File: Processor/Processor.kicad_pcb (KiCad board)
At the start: 2 copper layers, 100 x 100 mm, 44 parts, among them J1 Buss, J2 L2, J3 L3, U1 MC6800, U10 74LS573, U11 74LS573, U2 74LS74, U3 74LS00, U4 74LS245, U5 74LS573, U6 74LS138, U7 GAL20V8, U8 74LS04, U9 74LS573, Y1 2.0MHz

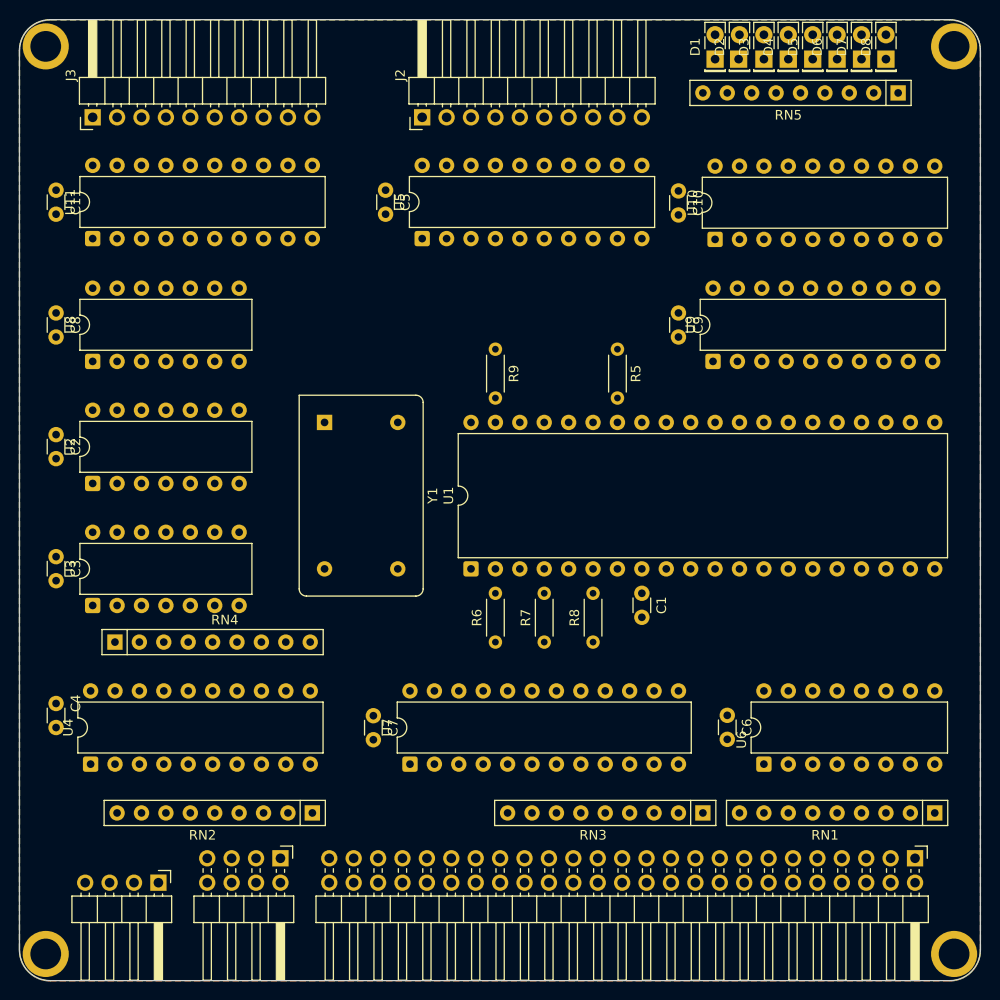
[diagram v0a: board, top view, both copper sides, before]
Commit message: a bunch of stuff
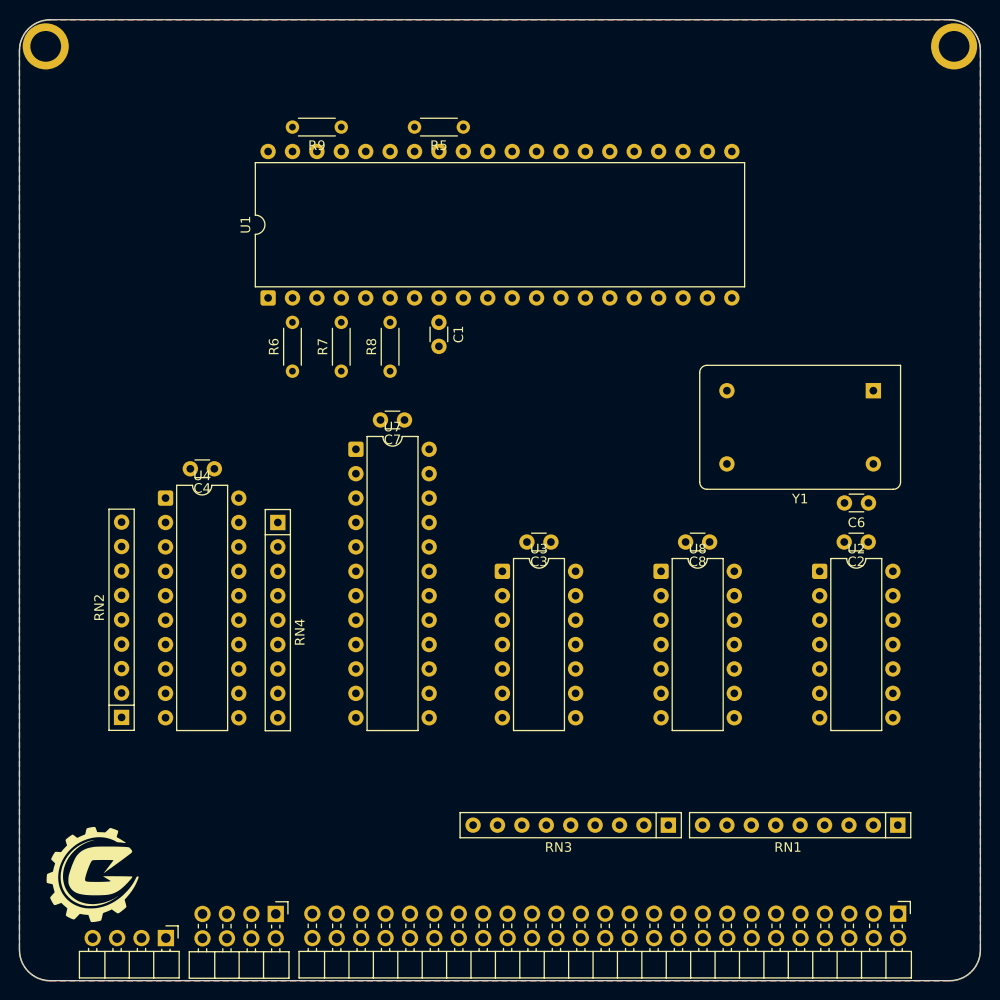
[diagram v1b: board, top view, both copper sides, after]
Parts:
- removed C10, C11, C5, C9: 100n, Capacitor_THT:C_Disc_D3.0mm_W1.6mm_P2.50mm
- removed D1: S0, LED_THT:LED_Rectangular_W5.0mm_H2.0mm
- removed D2: S1, LED_THT:LED_Rectangular_W5.0mm_H2.0mm
- removed D3: S2, LED_THT:LED_Rectangular_W5.0mm_H2.0mm
- removed D4: S3, LED_THT:LED_Rectangular_W5.0mm_H2.0mm
- removed D5: S4, LED_THT:LED_Rectangular_W5.0mm_H2.0mm
- removed D6: S5, LED_THT:LED_Rectangular_W5.0mm_H2.0mm
- removed D7: S6, LED_THT:LED_Rectangular_W5.0mm_H2.0mm
- removed D8: S7, LED_THT:LED_Rectangular_W5.0mm_H2.0mm
- removed J2: L2, Connector_PinHeader_2.54mm:PinHeader_1x10_P2.54mm_Horizontal
- removed J3: L3, Connector_PinHeader_2.54mm:PinHeader_1x10_P2.54mm_Horizontal
- removed RN5: 220Ω, Resistor_THT:R_Array_SIP9
- removed U10, U11, U5, U9: 74LS573, Package_DIP:DIP-20_W7.62mm
- removed U6: 74LS138, Package_DIP:DIP-16_W7.62mm
- added G1: Logo, 0-Footprints:Crank, F.Cu at (32.7, 114.0)
- U7: value GAL20V8 -> GAL22V10
- moved C2 85.3 mm to (113.3, 79.4), turned to 180 degrees
- moved U2 76.2 mm to (108.3, 82.4), turned to 0 degrees
- moved C8 72.1 mm to (96.8, 79.4), turned to 180 degrees
- moved U8 63.1 mm to (91.8, 82.4), turned to 0 degrees
- moved Y1 57.2 mm to (113.9, 63.6), turned to 180 degrees
- moved C3 51.5 mm to (80.3, 79.4), turned to 180 degrees
- moved U3 42.8 mm to (75.3, 82.4), turned to 0 degrees
- moved R6 35.2 mm to (53.4, 61.6)
- moved C1 35.2 mm to (68.7, 56.5)
- moved R7 35.2 mm to (58.5, 61.6)
- moved R8 35.2 mm to (63.6, 61.6)
- moved U1 35.2 mm to (50.9, 54.0)
- moved U7 33.2 mm to (60.0, 69.7), turned to 0 degrees
- moved C7 30.9 mm to (65.1, 66.7), turned to 180 degrees
- moved C4 29.5 mm to (45.3, 71.7), turned to 180 degrees
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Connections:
- J1 pad 10: BANK_0 -> unconnected-(J1-Pad10)
- J1 pad 12: BANK_1 -> unconnected-(J1-Pad12)
- J1 pad 14: BANK_2 -> unconnected-(J1-Pad14)
- J1 pad 16: BANK_3 -> unconnected-(J1-Pad16)
- J1 pad 18: BANK_4 -> unconnected-(J1-Pad18)
- J1 pad 20: BANK_5 -> unconnected-(J1-Pad20)
- J1 pad 22: BANK_6 -> unconnected-(J1-Pad22)
- J1 pad 24: BANK_7 -> unconnected-(J1-Pad24)
- J1 pad 44: Φ2 -> unconnected-(J1-Pad44)
- J1 pad B3: unconnected-(J1-PadB3) -> Φ2
- U3 pad 10: Net-(U6-O1) -> GND
- U3 pad 11: LOAD_0 -> unconnected-(U3-Pad11)
- U3 pad 12: Net-(U6-O0) -> GND
- U3 pad 13: Net-(U6-O0) -> GND
- U3 pad 8: LOAD_1 -> unconnected-(U3-Pad8)
- U3 pad 9: Net-(U6-O1) -> GND
- U7 pad 10: A12 -> A8
- U7 pad 11: A11 -> GND
- U7 pad 13: A10 -> GND
- U7 pad 14: A9 -> GND
- U7 pad 17: ~{LATCH_SEL} -> GND
- U7 pad 18: BUS_OK -> GND
- U7 pad 19: ~{IO_SEL} -> BUS_OK
- U7 pad 20: ~{BANK_SEL} -> ~{IO_SEL}
- U7 pad 21: ~{ROM_SEL} -> ~{BANK_SEL}
- U7 pad 22: ~{RAM_SEL} -> ~{ROM_SEL}
- U7 pad 23: A8 -> ~{RAM_SEL}
- U7 pad 3: GND -> A15
- U7 pad 4: GND -> A14
- U7 pad 5: GND -> A13
- U7 pad 6: GND -> A12
- U7 pad 7: A15 -> A11
- U7 pad 8: A14 -> A10
- U7 pad 9: A13 -> A9
- U8 pad 10: LOAD_2 -> unconnected-(U8-Pad10)
- U8 pad 11: Net-(U6-O2) -> GND
- U8 pad 12: LOAD_3 -> unconnected-(U8-Pad12)
- U8 pad 13: Net-(U6-O3) -> GND

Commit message: ordered v01 of the cpu
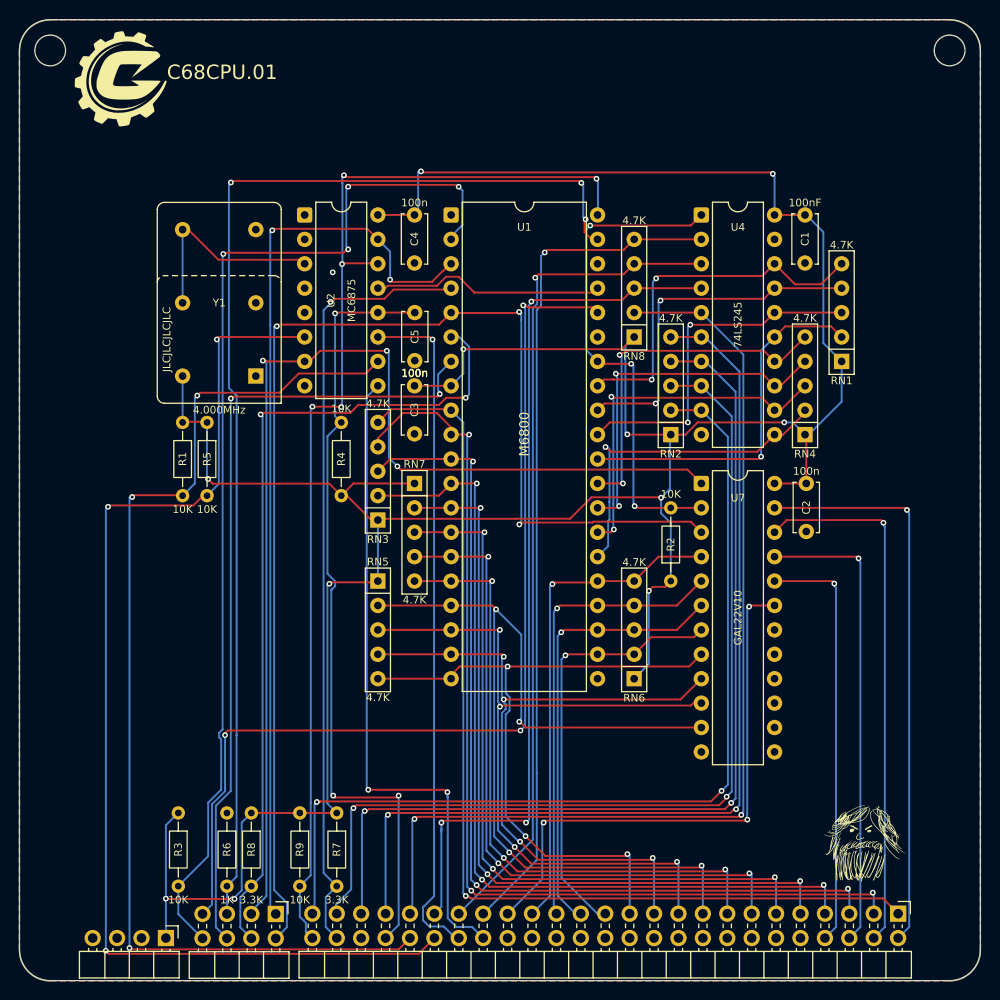
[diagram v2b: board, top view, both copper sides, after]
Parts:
- removed C6, C7, C8: 100n, Capacitor_THT:C_Disc_D3.0mm_W1.6mm_P2.50mm
- removed the R6 at (53.4, 61.6)
- removed U3: 74LS00, Package_DIP:DIP-14_W7.62mm
- removed U8: 74LS04, Package_DIP:DIP-14_W7.62mm
- added C5: 100n, 0-Footprints:C_Disc_D5.0mm_W2.5mm_P5.00mm, F.Cu at (66.1, 55.5)
- added G2: Crankery, 0-Footprints:crankery_small, F.Cu at (112.7, 110.8)
- added G3: Motorola, 0-Footprints:Motorola, B.Cu at (69.3, 31.0)
- added G4: Crank, 0-Footprints:Crank, B.Cu at (103.4, 31.1)
- added R1: 10K, 0-Footprints:R_Axial_DIN0204_L3.6mm_D1.6mm_P7.62mm_Horizontal, F.Cu at (42.0, 66.9)
- added R2: 10K, 0-Footprints:R_Axial_DIN0204_L3.6mm_D1.6mm_P7.62mm_Horizontal, F.Cu at (92.8, 83.4)
- added R3: 10K, 0-Footprints:R_Axial_DIN0204_L3.6mm_D1.6mm_P7.62mm_Horizontal, F.Cu at (41.5, 107.5)
- added R4: 10K, 0-Footprints:R_Axial_DIN0204_L3.6mm_D1.6mm_P7.62mm_Horizontal, F.Cu at (58.5, 74.5)
- added R9: 10K, 0-Footprints:R_Axial_DIN0204_L3.6mm_D1.6mm_P7.62mm_Horizontal, F.Cu at (54.2, 107.5)
- added RN5: 4.7K, 0-Footprints:R_Array_SIP5, F.Cu at (62.3, 83.4)
- added RN6: 4.7K, 0-Footprints:R_Array_SIP5, F.Cu at (89.0, 93.6)
- added RN7: 4.7K, 0-Footprints:R_Array_SIP5, F.Cu at (66.1, 73.3)
- added RN8: 4.7K, 0-Footprints:R_Array_SIP5, F.Cu at (89.0, 58.0)
- C1: value 100n -> 100nF; footprint Capacitor_THT:C_Disc_D3.0mm_W1.6mm_P2.50mm -> 0-Footprints:C_Disc_D5.0mm_W2.5mm_P5.00mm
- C2, C3, C4: footprint Capacitor_THT:C_Disc_D3.0mm_W1.6mm_P2.50mm -> 0-Footprints:C_Disc_D5.0mm_W2.5mm_P5.00mm
- G1: value Logo -> Crank
- R5, R7, R8: footprint Resistor_THT:R_Axial_DIN0204_L3.6mm_D1.6mm_P5.08mm_Horizontal -> 0-Footprints:R_Axial_DIN0204_L3.6mm_D1.6mm_P7.62mm_Horizontal
- R6: renamed from R9; footprint Resistor_THT:R_Axial_DIN0204_L3.6mm_D1.6mm_P5.08mm_Horizontal -> 0-Footprints:R_Axial_DIN0204_L3.6mm_D1.6mm_P7.62mm_Horizontal
- RN1, RN2, RN3, RN4: footprint Resistor_THT:R_Array_SIP9 -> 0-Footprints:R_Array_SIP5
- U1: value MC6800 -> M6800; footprint Package_DIP:DIP-40_W15.24mm -> 0-Footprints:DIP-40_W15.24mm
- U2: value 74LS74 -> MC6875; footprint Package_DIP:DIP-14_W7.62mm -> 0-Footprints:DIP-16_W7.62mm
- U4: footprint Package_DIP:DIP-20_W7.62mm -> 0-Footprints:DIP-20_W7.62mm
- U7: footprint Package_DIP:DIP-24_W7.62mm -> 0-Footprints:DIP-24_W7.62mm
- Y1: value 2.0MHz -> 4.000MHz; footprint Oscillator:Oscillator_DIP-14 -> 0-Footprints:Oscillator_DIP-14
- moved G1 82.9 mm to (35.6, 31.2)
- moved R6 72.4 mm to (46.6, 107.5), turned to -90 degrees
- moved U2 65.2 mm to (54.7, 45.3)
- moved RN2 64.3 mm to (92.8, 68.2)
- moved Y1 64.3 mm to (49.6, 62.1), turned to 90 degrees
- moved U4 63.1 mm to (96.0, 45.3)
- moved RN4 55.6 mm to (106.8, 68.2), turned to 90 degrees
- moved RN1 48.6 mm to (110.6, 60.6), turned to 90 degrees
- moved R8 48.2 mm to (49.1, 107.5), turned to -90 degrees
- moved R7 46.0 mm to (58.0, 107.5), turned to -90 degrees
- moved RN3 43.8 mm to (62.3, 77.1), turned to 90 degrees
- moved R5 40.7 mm to (44.5, 66.9), turned to -90 degrees
- moved C1 38.6 mm to (106.8, 50.3), turned to 90 degrees
- moved U7 36.1 mm to (96.0, 73.3)
- moved C4 29.9 mm to (66.1, 50.3), turned to 90 degrees
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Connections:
- net 2.0MHz renamed Net-(U2-EXT_IN)
- C1 pad 1: +5V -> GND
- C1 pad 2: GND -> +5V
- C2 pad 1: +5V -> GND
- C2 pad 2: GND -> +5V
- C3 pad 1: +5V -> GND
- C3 pad 2: GND -> +5V
- C4 pad 1: +5V -> GND
- C4 pad 2: GND -> +5V
- J1 pad 36: unconnected-(J1-Pad36) -> MEM_CLK
- J1 pad 38: unconnected-(J1-Pad38) -> DMA_GRANT
- J1 pad 40: unconnected-(J1-Pad40) -> MEMRDY
- J1 pad 42: unconnected-(J1-Pad42) -> ~{DMA_REQ}
- J1 pad 44: unconnected-(J1-Pad44) -> ~{POR}
- J1 pad P1: (no net) -> +5V
- J1 pad P2: (no net) -> GND
- J1 pad P3: (no net) -> unconnected-(J1-+12V-PadP3)
- J1 pad P4: (no net) -> unconnected-(J1--12V-PadP4)
- R5 pad 2: R/~{W} -> MEMRDY
- RN1 pad 2: A0 -> D3
- RN1 pad 3: A1 -> D2
- RN1 pad 4: A2 -> D1
- RN1 pad 5: A3 -> D0
- RN3 pad 2: A8 -> A3
- RN3 pad 3: A9 -> A2
- RN3 pad 4: A10 -> A1
- RN3 pad 5: A11 -> A0
- RN4 pad 2: D0 -> D7
- RN4 pad 3: D1 -> D6
- RN4 pad 4: D2 -> D5
- RN4 pad 5: D3 -> D4
- U1 pad 36: ~{DBE} -> DBE
- U1 pad 37: Φ2 -> Net-(U1-Phi2)
- U2 pad 1: +5V -> GND
- U2 pad 10: GND -> ~{DMA_REQ}
- U2 pad 11: GND -> DMA_GRANT
- U2 pad 12: GND -> ~{POR}
- U2 pad 13: GND -> Net-(U1-Phi2)
- U2 pad 14: +5V -> ~{RESET}
- U2 pad 2: CLK_B -> unconnected-(U2-X2-Pad2)
- U2 pad 4: +5V -> unconnected-(U2-4x_fo-Pad4)
- U2 pad 5: CLK_A -> unconnected-(U2-2x_fo-Pad5)
- U2 pad 6: CLK_B -> MEMRDY
- U2 pad 7: GND -> Φ2
- U2 pad 8: unconnected-(U2B-~{Q}-Pad8) -> GND
- U2 pad 9: unconnected-(U2B-Q-Pad9) -> MEM_CLK
- U7 pad 10: A8 -> A9
- U7 pad 11: GND -> A8
- U7 pad 3: A15 -> VMA
- U7 pad 4: A14 -> A15
- U7 pad 5: A13 -> A14
- U7 pad 6: A12 -> A13
- U7 pad 7: A11 -> A12
- U7 pad 8: A10 -> A11
- U7 pad 9: A9 -> A10
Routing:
- net +5V: track 0.00 -> 315.9 mm, vias 0 -> 11
- net VMA: track 0.00 -> 132.8 mm, vias 0 -> 3
- net ~{TSC}: track 0.00 -> 120.0 mm, vias 0 -> 3
- net MEMRDY: track 0.00 -> 118.3 mm, vias 0 -> 3
- net ~{RESET}: track 0.00 -> 118.0 mm, vias 0 -> 5
- net Φ2: track 0.00 -> 115.9 mm, vias 0 -> 3
- net ~{DMA_REQ}: track 0.00 -> 113.6 mm, vias 0 -> 3
- net ~{HALT}: track 0.00 -> 111.8 mm, vias 0 -> 4
- net BD3: track 0.00 -> 105.5 mm, vias 0 -> 2
- net A1: track 0.00 -> 105.0 mm, vias 0 -> 3
- net A0: track 0.00 -> 105.0 mm, vias 0 -> 1
- net DBE: track 0.00 -> 103.2 mm, vias 0 -> 3
- net BD4: track 0.00 -> 100.8 mm, vias 0 -> 2
- net BD5: track 0.00 -> 99.8 mm, vias 0 -> 2
- net BD6: track 0.00 -> 98.5 mm, vias 0 -> 2
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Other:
- board text added: "C68 CPU"
- board text added: "C68CPU.01"
- board text added: "Crankery - April 2026 - Dave Hamilton"
- board text added: "JLCJLCJLCJLC"
- board text added: "Motorola M6800"
